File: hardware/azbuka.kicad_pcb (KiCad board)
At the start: 2 copper layers, 15 parts, among them IC1 ATTINY85-S, P1 USB_OTG, P2 CONN_01X06, Q1 MOSFET_P_CH, U3 SJ1-3524NG

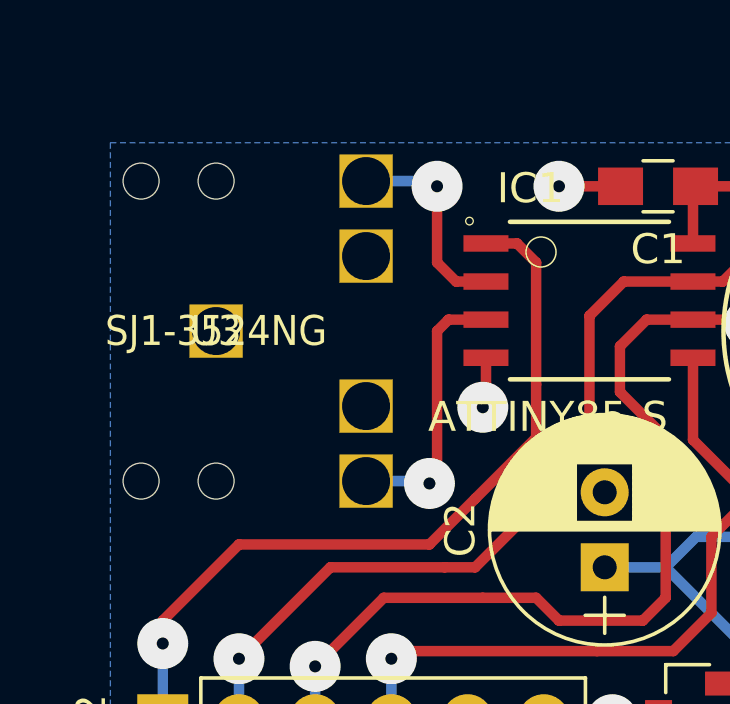
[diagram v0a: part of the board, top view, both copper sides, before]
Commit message: Version 3 completed.
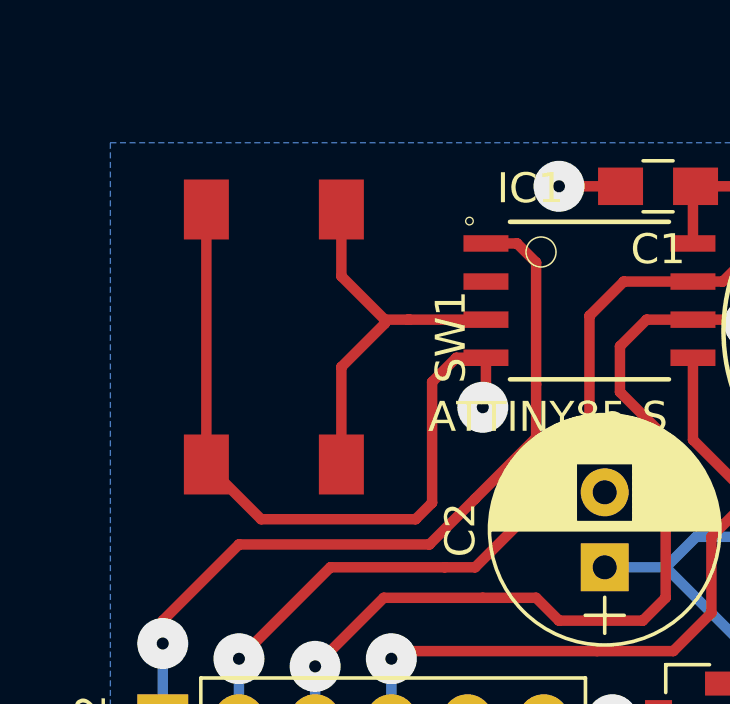
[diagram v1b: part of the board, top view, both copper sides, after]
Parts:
- removed U3: SJ1-3524NG, azbuka:PIN-4_MODIFIED_NO_HOLES
- added SW1: TACT-SWITCH, azbuka:SMD_RED_TACTILE_SWITCH, F.Cu at (130.4, 65.5)
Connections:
- IC1 pad 2: DAH -> Net-(IC1-Pad2)
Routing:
- net GND: track 23.8 -> 46.9 mm
- net DAH: track 6.87 -> 0.00 mm, vias 1 -> 0
- net DIT: track 9.12 -> 13.1 mm, vias 1 -> 0
